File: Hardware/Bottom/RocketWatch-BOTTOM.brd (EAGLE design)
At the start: 33 x 33 mm, 32 parts, among them U1 AD5242-SO16

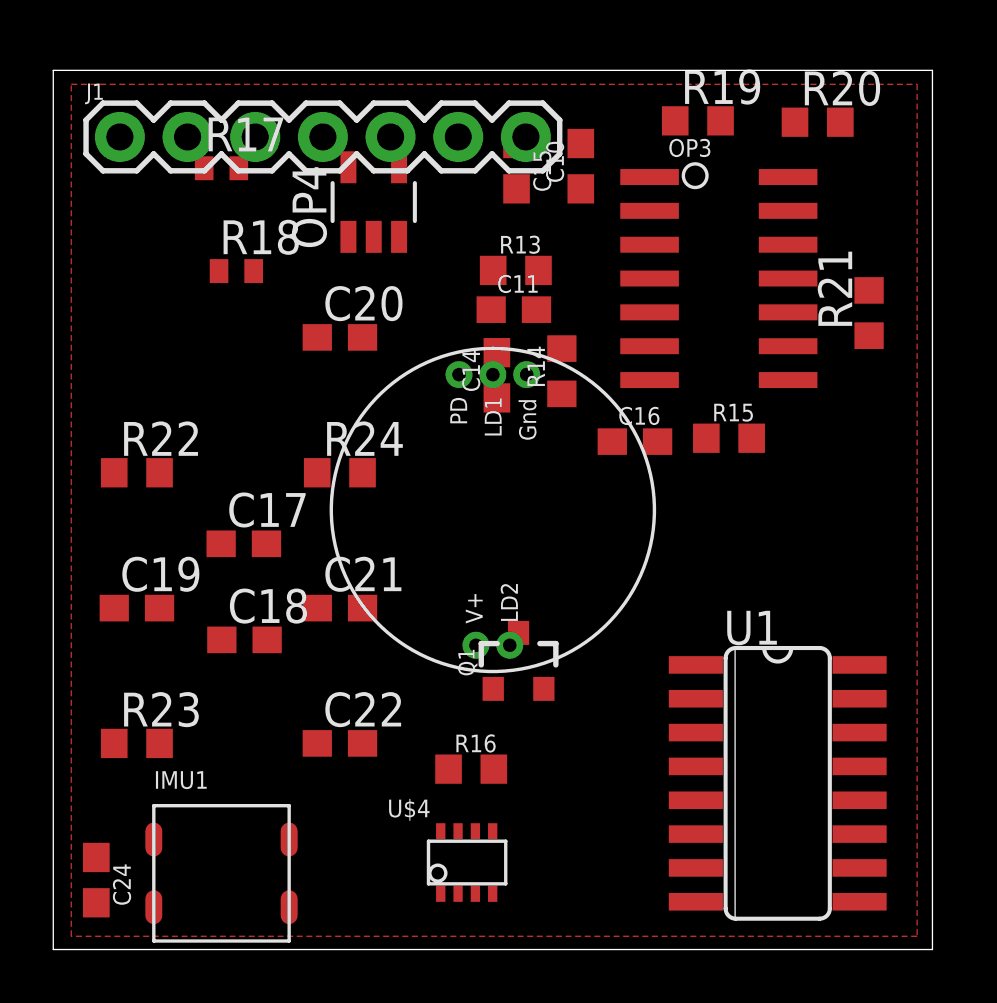
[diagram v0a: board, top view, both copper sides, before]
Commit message: most of the bottom board routed. Few things left to route and clean up to show all labels.
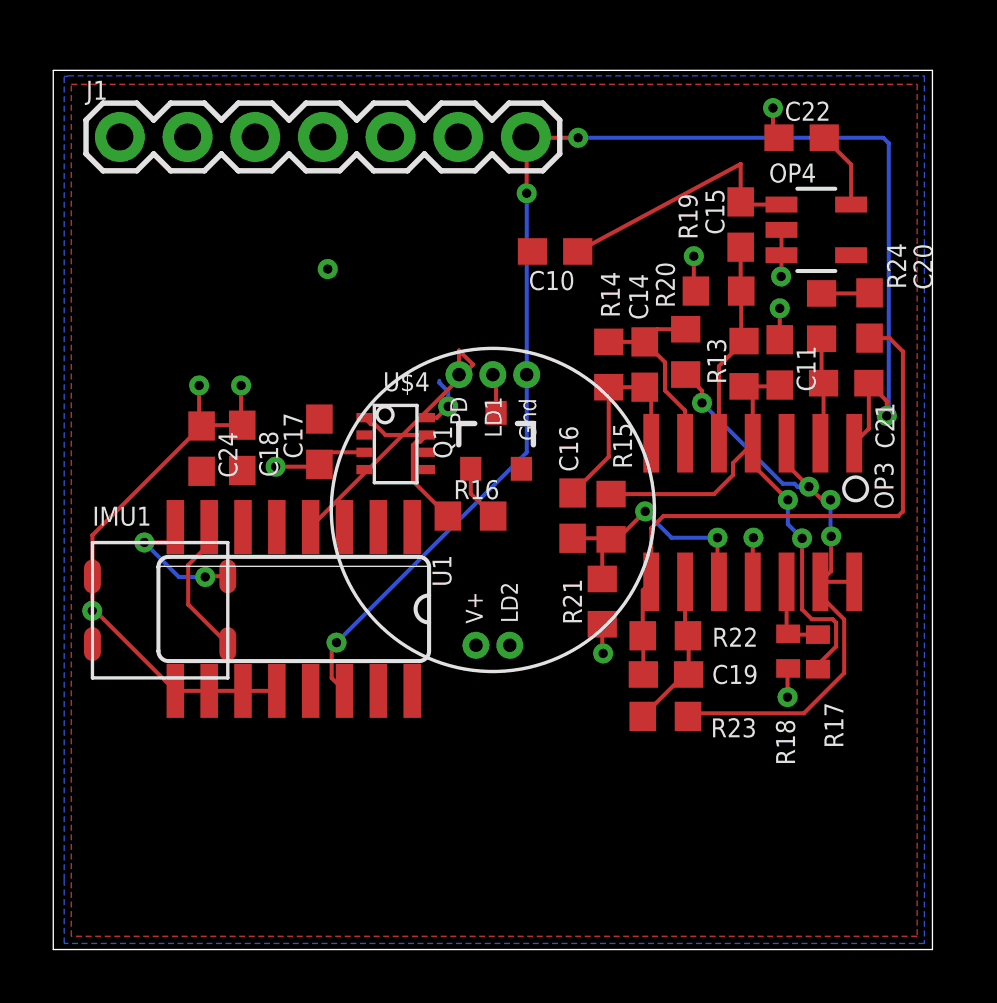
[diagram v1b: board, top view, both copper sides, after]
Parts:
- moved R17 28.8 mm to (31.2, 13.7), turned to 270 degrees
- moved C22 28.6 mm to (30.6, 33.0)
- moved R18 25.1 mm to (30.1, 13.7), turned to 90 degrees
- moved C21 20.8 mm to (32.3, 23.8)
- moved R22 20.8 mm to (25.5, 14.3), turned to 180 degrees
- moved C19 20.0 mm to (25.5, 12.8)
- moved C20 19.9 mm to (33.1, 26.3), turned to 90 degrees
- moved R23 19.9 mm to (25.5, 11.3), turned to 180 degrees
- moved U1 19.3 mm to (11.5, 15.3), turned to 180 degrees
- moved R24 19.0 mm to (31.3, 26.3), turned to 90 degrees
- moved C24 16.7 mm to (8.07, 21.3)
- moved OP4 16.6 mm to (31.1, 29.5), turned to 270 degrees
- moved U$4 15.9 mm to (15.4, 21.5), turned to 270 degrees
- moved R21 14.8 mm to (23.1, 15.6)
- moved C11 10.2 mm to (29.8, 24.5), turned to 270 degrees
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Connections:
- removed net LED: Q1.3
- net LED.C: now also Q1.3
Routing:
- net A7/PPG: track 0.00 -> 52.0 mm, vias 0 -> 4
- net GND: track 0.00 -> 34.0 mm, vias 0 -> 11
- net VREF: track 0.00 -> 24.5 mm, vias 0 -> 4
- net 3.3V: track 0.00 -> 23.4 mm, vias 0 -> 2
- net N$19: track 0.00 -> 22.8 mm
- net PD.C: track 0.00 -> 10.3 mm
- net A6/TIA: track 0.00 -> 9.94 mm
- net N$17: track 0.00 -> 9.62 mm, vias 0 -> 2
- net N$16: track 0.00 -> 8.09 mm
- net N$13: track 0.00 -> 7.80 mm
- net N$15: track 0.00 -> 7.52 mm
- net N$9: track 0.00 -> 6.51 mm
- net N$18: track 0.00 -> 5.91 mm
- net SDA: track 0.00 -> 5.62 mm, vias 0 -> 2
- net SCL: track 0.00 -> 5.33 mm
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- added copper zone on layer 16, net GND
